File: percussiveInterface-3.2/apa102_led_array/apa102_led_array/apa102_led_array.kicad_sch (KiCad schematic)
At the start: 49 parts

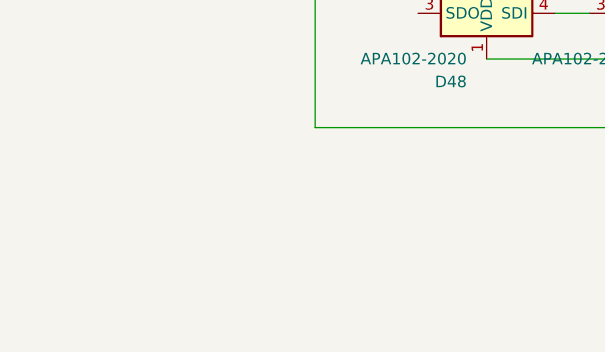
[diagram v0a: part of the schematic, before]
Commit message: many changes
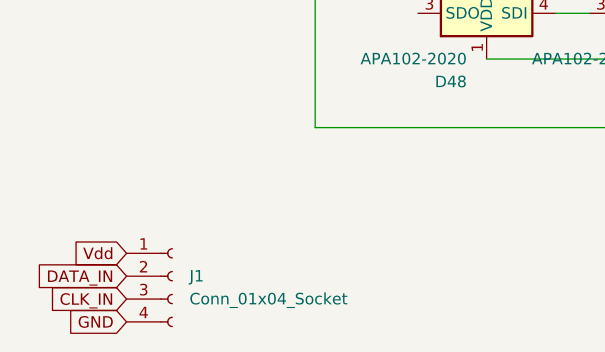
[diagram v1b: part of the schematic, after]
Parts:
- added J1: Conn_01x04_Socket, Connector_Pin:Pin_D0.7mm_L6.5mm_W1.8mm_FlatFork, symbol Connector:Conn_01x04_Socket
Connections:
- net CLK_IN: now also J1.3 (Pin_3)
- net DATA_IN: now also J1.2 (Pin_2)
- net GND: now also J1.4 (Pin_4)
- net Vdd: now also J1.1 (Pin_1)
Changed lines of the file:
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@@
+    (stroke (width 0) (type default))
+  )
+  (wire (pts (xy 78.74 58.42) (xy 72.39 58.42))
+    (stroke (width 0) (type default))
+  )
+  (wire (pts (xy 142.24 106.68) (xy 160.02 106.68))
+    (stroke (width 0) (type default))
+  )
+  (wire (pts (xy 86.36 88.9) (xy 86.36 91.44))
+    (stroke (width 0) (type default))
+  )
+  (wire (pts (xy 220.98 81.28) (xy 224.79 81.28))
+    (stroke (width 0) (type default))
+  )
+  (wire (pts (xy 139.7 129.54) (xy 157.48 129.54))
+    (stroke (width 0) (type default))
+  )
+  (wire (pts (xy 93.98 58.42) (xy 97.79 58.42))
+    (stroke (width 0) (type default))
+  )
+  (wire (pts (xy 201.93 81.28) (xy 205.74 81.28))
+    (stroke (width 0) (type default))
+  )
+  (wire (pts (xy 67.31 132.08) (xy 68.58 132.08))
+    (stroke (width 0) (type default))
+  )
+  (wire (pts (xy 175.26 129.54) (xy 194.31 129.54))
+    (stroke (width 0) (type default))
+  )
+  (wire (pts (xy 105.41 132.08) (xy 124.46 132.08))
+    (stroke (width 0) (type default))
+  )
+  (wire (pts (xy 226.06 119.38) (xy 226.06 142.24))
+    (stroke (width 0) (type default))
+  )
+  (wire (pts (xy 201.93 40.64) (xy 205.74 40.64))
+    (stroke (width 0) (type default))
+  )
+  (wire (pts (xy 132.08 142.24) (xy 134.62 142.24))
+    (stroke (width 0) (type default))
+  )
+  (wire (pts (xy 129.54 40.64) (xy 132.08 40.64))
+    (stroke (width 0) (type default))
+  )
+  (wire (pts (xy 86.36 50.8) (xy 105.41 50.8))
+    (stroke (width 0) (type default))
+  )
+  (wire (pts (xy 129.54 38.1) (xy 132.08 38.1))
+    (stroke (width 0) (type default))
+  )
+  (wire (pts (xy 73.66 99.06) (xy 73.66 121.92))
+    (stroke (width 0) (type default))
+  )
+  (wire (pts (xy 93.98 101.6) (xy 97.79 101.6))
+    (stroke (width 0) (type default))
+  )
+  (wire (pts (xy 165.1 40.64) (xy 167.64 40.64))
+    (stroke (width 0) (type default))
+  )
+  (wire (pts (xy 220.98 78.74) (xy 226.06 78.74))
+    (stroke (width 0) (type default))
+  )
+  (wire (pts (xy 185.42 139.7) (xy 187.96 139.7))
+    (stroke (width 0) (type default))
+  )
+  (wire (pts (xy 157.48 114.3) (xy 139.7 114.3))
+    (stroke (width 0) (type default))
+  )
+  (wire (pts (xy 78.74 78.74) (xy 73.66 78.74))
+    (stroke (width 0) (type default))
+  )
+  (wire (pts (xy 104.14 114.3) (xy 86.36 114.3))
+    (stroke (width 0) (type default))
+  )
+  (wire (pts (xy 149.86 142.24) (xy 152.4 142.24))
+    (stroke (width 0) (type default))
+  )
+  (wire (pts (xy 142.24 147.32) (xy 160.02 147.32))
+    (stroke (width 0) (type default))
+  )
+  (wire (pts (xy 213.36 66.04) (xy 213.36 73.66))
+    (stroke (width 0) (type default))
+  )
+  (wire (pts (xy 104.14 129.54) (xy 121.92 129.54))
+    (stroke (width 0) (type default))
+  )
+  (wire (pts (xy 175.26 48.26) (xy 194.31 48.26))
+    (stroke (width 0) (type default))
+  )
+  (wire (pts (xy 132.08 60.96) (xy 134.62 60.96))
+    (stroke (width 0) (type default))
+  )
+  (wire (pts (xy 195.58 66.04) (xy 213.36 66.04))
     (stroke (width 0) (type default))
   )
@@
     (stroke (width 0) (type default))
   )
-  (wire (pts (xy 78.74 58.42) (xy 72.39 58.42))
-    (stroke (width 0) (type default))
-  )
-  (wire (pts (xy 142.24 106.68) (xy 160.02 106.68))
-    (stroke (width 0) (type default))
-  )
-  (wire (pts (xy 86.36 88.9) (xy 86.36 91.44))
-    (stroke (width 0) (type default))
-  )
-  (wire (pts (xy 220.98 81.28) (xy 224.79 81.28))
-    (stroke (width 0) (type default))
-  )
-  (wire (pts (xy 139.7 129.54) (xy 157.48 129.54))
-    (stroke (width 0) (type default))
-  )
-  (wire (pts (xy 93.98 58.42) (xy 97.79 58.42))
-    (stroke (width 0) (type default))
-  )
-  (wire (pts (xy 201.93 81.28) (xy 205.74 81.28))
-    (stroke (width 0) (type default))
-  )
-  (wire (pts (xy 67.31 132.08) (xy 68.58 132.08))
-    (stroke (width 0) (type default))
-  )
-  (wire (pts (xy 175.26 129.54) (xy 194.31 129.54))
-    (stroke (width 0) (type default))
-  )
-  (wire (pts (xy 105.41 132.08) (xy 124.46 132.08))
-    (stroke (width 0) (type default))
-  )
-  (wire (pts (xy 226.06 119.38) (xy 226.06 142.24))
-    (stroke (width 0) (type default))
-  )
-  (wire (pts (xy 201.93 40.64) (xy 205.74 40.64))
-    (stroke (width 0) (type default))
-  )
-  (wire (pts (xy 132.08 142.24) (xy 134.62 142.24))
-    (stroke (width 0) (type default))
-  )
-  (wire (pts (xy 129.54 40.64) (xy 132.08 40.64))
-    (stroke (width 0) (type default))
-  )
-  (wire (pts (xy 86.36 50.8) (xy 105.41 50.8))
-    (stroke (width 0) (type default))
-  )
-  (wire (pts (xy 129.54 38.1) (xy 132.08 38.1))
-    (stroke (width 0) (type default))
-  )
-  (wire (pts (xy 73.66 99.06) (xy 73.66 121.92))
-    (stroke (width 0) (type default))
-  )
-  (wire (pts (xy 93.98 101.6) (xy 97.79 101.6))
-    (stroke (width 0) (type default))
-  )
-  (wire (pts (xy 165.1 40.64) (xy 167.64 40.64))
-    (stroke (width 0) (type default))
-  )
-  (wire (pts (xy 220.98 78.74) (xy 226.06 78.74))
-    (stroke (width 0) (type default))
-  )
-  (wire (pts (xy 185.42 139.7) (xy 187.96 139.7))
-    (stroke (width 0) (type default))
-  )
-  (wire (pts (xy 157.48 114.3) (xy 139.7 114.3))
-    (stroke (width 0) (type default))
-  )
-  (wire (pts (xy 78.74 78.74) (xy 73.66 78.74))
-    (stroke (width 0) (type default))
-  )
-  (wire (pts (xy 104.14 114.3) (xy 86.36 114.3))
-    (stroke (width 0) (type default))
-  )
-  (wire (pts (xy 149.86 142.24) (xy 152.4 142.24))
-    (stroke (width 0) (type default))
-  )
-  (wire (pts (xy 142.24 147.32) (xy 160.02 147.32))
-    (stroke (width 0) (type default))
-  )
-  (wire (pts (xy 213.36 66.04) (xy 213.36 73.66))
-    (stroke (width 0) (type default))
-  )
-  (wire (pts (xy 104.14 129.54) (xy 121.92 129.54))
-    (stroke (width 0) (type default))
-  )
-  (wire (pts (xy 175.26 48.26) (xy 194.31 48.26))
-    (stroke (width 0) (type default))
-  )
-  (wire (pts (xy 132.08 60.96) (xy 134.62 60.96))
-    (stroke (width 0) (type default))
-  )
-  (wire (pts (xy 195.58 66.04) (xy 213.36 66.04))
-    (stroke (width 0) (type default))
-  )
   (wire (pts (xy 139.7 33.02) (xy 157.48 33.02))
     (stroke (width 0) (type default))
@@
   (wire (pts (xy 203.2 142.24) (xy 205.74 142.24))
     (stroke (width 0) (type default))
+  )
+  (global_label "GND" (shape input) (at 46.355 176.53 180) (fields_autoplaced)
+    (effects (font (size 1.27 1.27)) (justify right))
+    (property "Intersheetrefs" "${INTERSHEET_REFS}" (at 39.4993 176.53 0)
+      (effects (font (size 1.27 1.27)) (justify right) hide)
+    )
+  )
+  (global_label "Vdd" (shape input) (at 46.355 168.91 180) (fields_autoplaced)
+    (effects (font (size 1.27 1.27)) (justify right))
+    (property "Intersheetrefs" "${INTERSHEET_REFS}" (at 39.9832 168.91 0)
+      (effects (font (size 1.27 1.27)) (justify right) hide)
+    )
+  )
+  (global_label "CLK_IN" (shape input) (at 46.355 173.99 180) (fields_autoplaced)
+    (effects (font (size 1.27 1.27)) (justify right))
+    (property "Intersheetrefs" "${INTERSHEET_REFS}" (at 36.8988 173.99 0)
+      (effects (font (size 1.27 1.27)) (justify right) hide)
+    )
   )
   (global_label "DATA_IN" (shape input) (at 66.04 38.1 180) (fields_autoplaced)
@@
     )
   )
+  (global_label "DATA_IN" (shape input) (at 46.355 171.45 180) (fields_autoplaced)
+    (effects (font (size 1.27 1.27)) (justify right))
+    (property "Intersheetrefs" "${INTERSHEET_REFS}" (at 36.0521 171.45 0)
+      (effects (font (size 1.27 1.27)) (justify right) hide)
+    )
+  )
   (global_label "Vdd" (shape input) (at 247.65 147.32 0) (fields_autoplaced)
     (effects (font (size 1.27 1.27)) (justify left))
@@
         )
       )
+    )
+  )
+  (symbol (lib_id "Connector:Conn_01x04_Socket") (at 51.435 171.45 0) (unit 1)
+    (in_bom yes) (on_board yes) (dnp no) (fields_autoplaced)
+    (property "Reference" "J1" (at 53.34 171.45 0)
+      (effects (font (size 1.27 1.27)) (justify left))
+    )
+    (property "Value" "Conn_01x04_Socket" (at 53.34 173.99 0)
+      (effects (font (size 1.27 1.27)) (justify left))
+    )
+    (property "Footprint" "Connector_Pin:Pin_D0.7mm_L6.5mm_W1.8mm_FlatFork" (at 51.435 171.45 0)
+      (effects (font (size 1.27 1.27)) hide)
+    )
+    (property "Datasheet" "~" (at 51.435 171.45 0)
+      (effects (font (size 1.27 1.27)) hide)
+    )
+    (pin "1")
+    (pin "2")
+    (pin "3")
+    (pin "4")
+    (instances
+      (project "apa102_led_array"
+        (path "/09de0c71-f69c-4ec3-b98e-304a8f538cb4"
+          (reference "J1") (unit 1)
+        )
+      )
